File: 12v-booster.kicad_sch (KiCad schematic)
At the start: 21 parts, among them J201 12V_OUT, U202 MPM3810GQB-33, U203 TPS61089RNRR

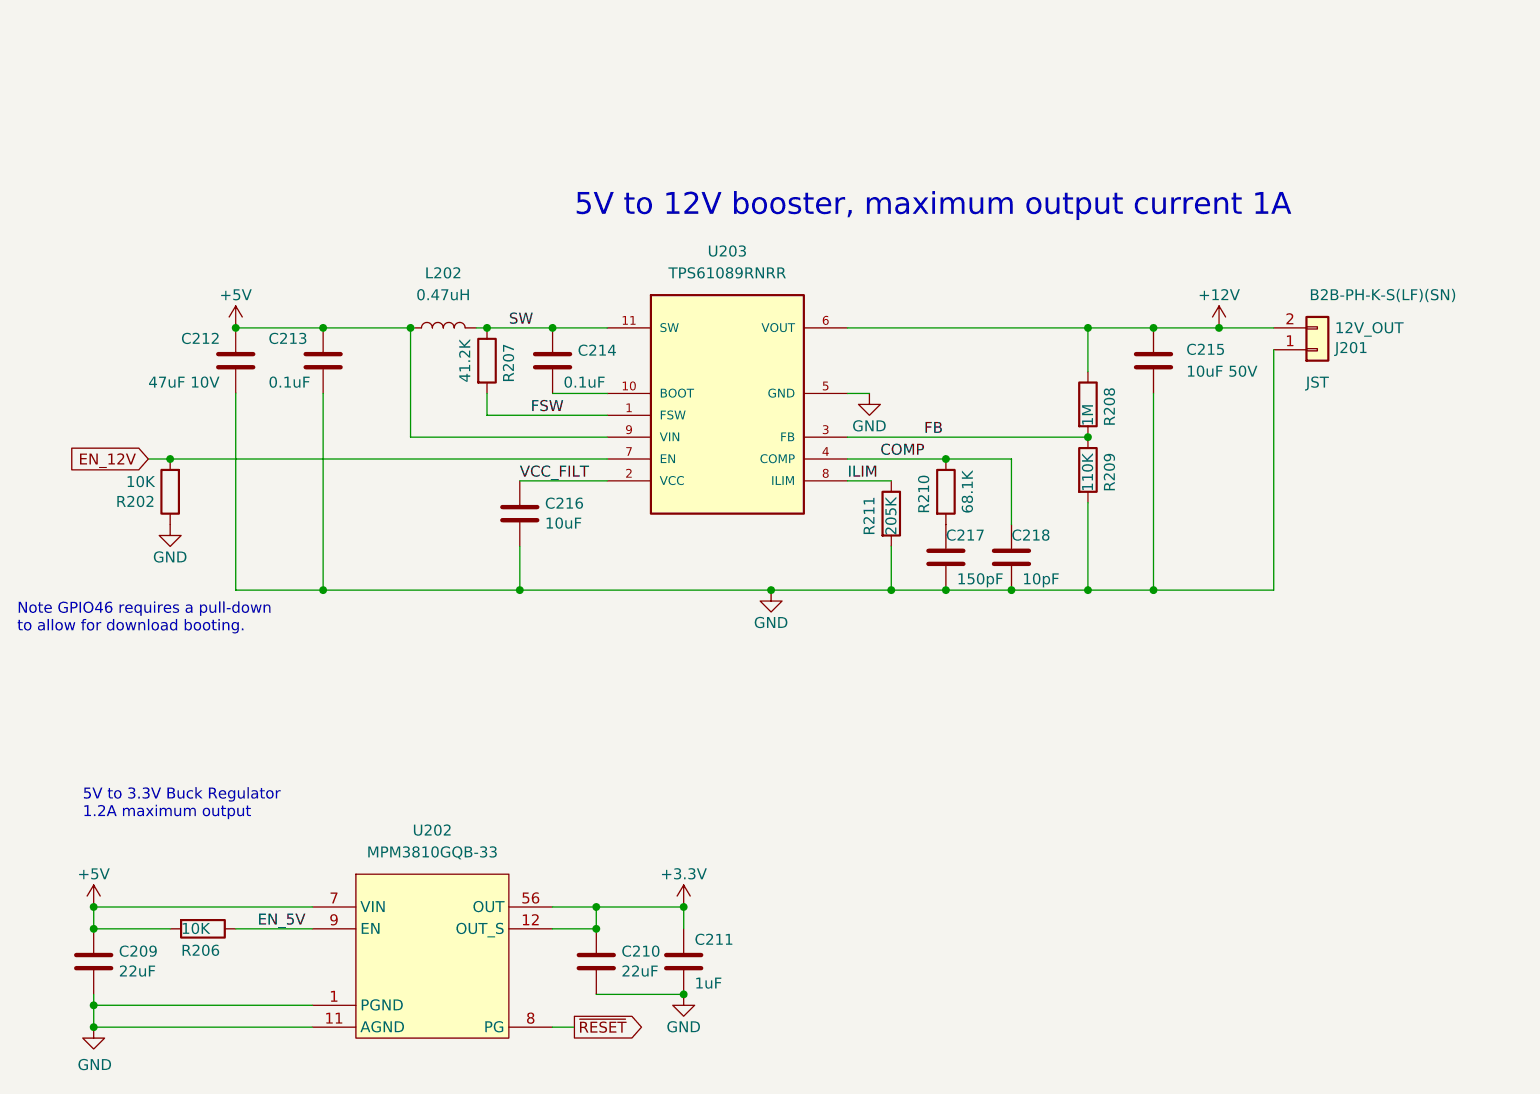
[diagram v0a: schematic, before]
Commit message: Latest 4.0 settings for pcbway
Signed-off-by: Aaron Williams <aaron.w2@gmail.com>
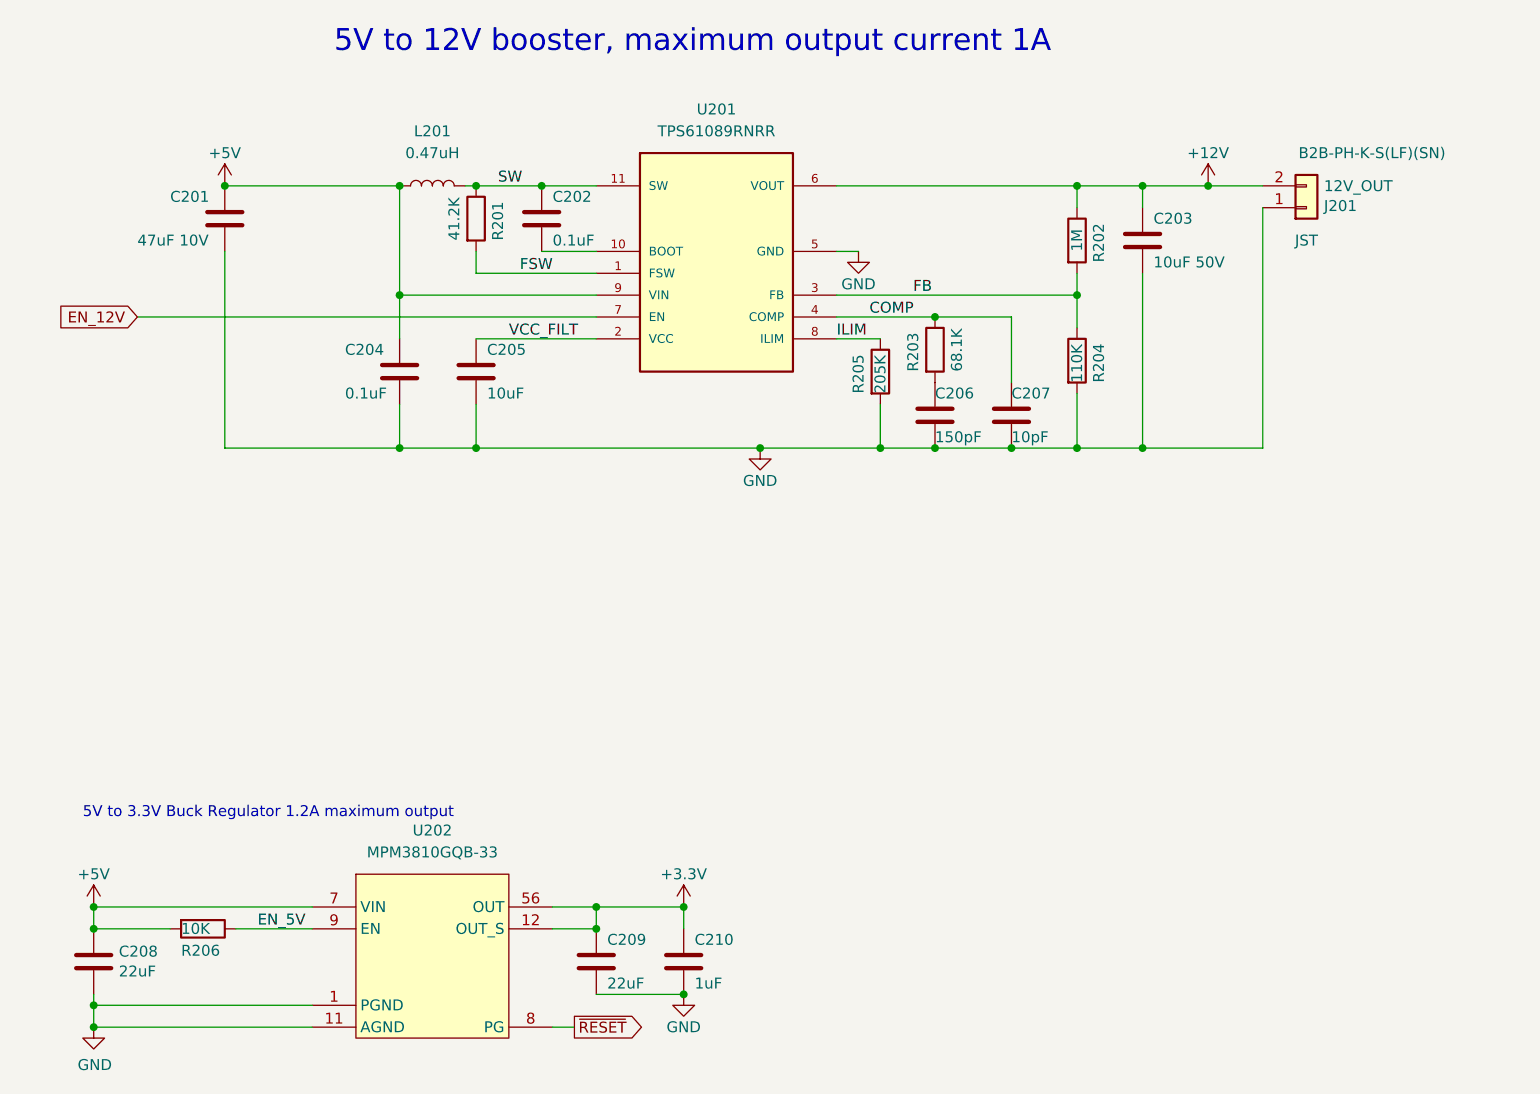
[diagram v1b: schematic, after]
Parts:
- removed R202: 10K, Resistor_SMD:R_0402_1005Metric, symbol Device:R
- C201: renamed from C212; SPN (none) -> 490-9961-1-ND; SPR (none) -> Digikey; SPURL (none) -> https://www.digikey.com/en/products/detail/murata-electroni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
- C203: renamed from C215; MFR (none) -> Murata Electronics; MPN (none) -> GRM21BR61H106KE43L; SPN (none) -> 490-18663-1-ND; SPR (none) -> Digikey; SPURL (none) -> https://www.digikey.com/en/products/detail/murata-electroni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
- C208: renamed from C209; DESC CAP CER 22UF 16V X5R 0603 -> 22 µF ±20% 16V Ceramic Capacitor X5R 0603 (1608 Metric); DK_Datasheet_Link (none) -> https://media.digikey.com/pdf/Data%20Sheets/Samsung%20PDFs/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; DK_Detail_Page (none) -> https://www.digikey.com/en/products/detail/samsung-electro-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; Digi-Key_PN (none) -> 1276-7076-1-ND; MANUFACTURER (none) -> Samsung Electro-Mechanics; Manufacturer (none) -> Samsung Electro-Mechanics; SPURL https://www.digikey.com/products/en/capacitors/ceramic-capa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 -> https://www.digikey.com/en/products/detail/samsung-electro-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
- C209: renamed from C210; DESC CAP CER 22UF 16V X5R 0603 -> 22 µF ±20% 16V Ceramic Capacitor X5R 0603 (1608 Metric); DK_Datasheet_Link (none) -> https://media.digikey.com/pdf/Data%20Sheets/Samsung%20PDFs/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; DK_Detail_Page (none) -> https://www.digikey.com/en/products/detail/samsung-electro-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; Digi-Key_PN (none) -> 1276-7076-1-ND; MANUFACTURER (none) -> Samsung Electro-Mechanics; Manufacturer (none) -> Samsung Electro-Mechanics; SPURL https://www.digikey.com/products/en/capacitors/ceramic-capa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 -> https://www.digikey.com/en/products/detail/samsung-electro-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
- C210: renamed from C211; DESC (none) -> CAP CER 1UF 25V X5R 0402; Digi-Key_PN (none) -> 490-GRM155R61E105MA12JCT-ND; MANUFACTURER (none) -> Murata Electronics; MFR (none) -> Murata Electronics; MPN (none) -> GRM155R61E105MA12J; Manufacturer (none) -> Murata Electronics; Manufacturer Part Number (none) -> GRM155R61E105MA12J; SPN (none) -> 490-GRM155R61E105MA12JCT-ND; SPURL (none) -> https://www.digikey.com/en/products/detail/murata-electroni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
- L201: renamed from L202; DESC (none) -> 470 nH Shielded Drum Core, Wirewound Inductor 7 A 19.2mOhm 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; DK_Datasheet_Link (none) -> https://www.bourns.com/docs/product-datasheets/srp3212.pdf; DK_Detail_Page (none) -> https://www.bourns.com/docs/product-datasheets/srp3212.pdf; Digi-Key_PN (none) -> 118-SRP3212-R47MCT-ND; MFR (none) -> Bourns Inc.; MPN (none) -> SRP3212-R47M; Manufacturer (none) -> Bourns Inc.; Manufacturer Part Number (none) -> SRP3212-R47M; SPN (none) -> 118-SRP3212-R47MCT-ND; SPR (none) -> Digikey; SPURL (none) -> https://www.bourns.com/docs/product-datasheets/srp3212.pdf; Status (none) -> Active
- R201: renamed from R207; SPN 541-2979-1-ND -> (none); SPR Digikey -> (none); SPURL https://www.digikey.com/products/en?keywords=541-2979-1-ND -> (none)
- R204: renamed from R209; DESC 100 kOhms ±1% 0.063W, 1/16W Chip Resistor 0402 (1005 Metric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 -> (none); MFR YAGEO -> (none); MPN RC0402FR-07100KL -> (none); SPN 311-100KLRCT-ND -> (none); SPR Digikey -> (none)
- R206: DESC (none) -> 10 kOhms ±1% 0.063W, 1/16W Chip Resistor 0402 (1005 Metric)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; Digi-Key_PN (none) -> 311-10.0KLRCT-ND; MANUFACTURER (none) -> YAGEO; MFR (none) -> YAGEO; MPN (none) -> RC0402FR-0710KL; Manufacturer (none) -> YAGEO; Manufacturer Part Number (none) -> RC0402FR-0710KL; SPN 541-2979-1-ND -> 311-10.0KLRCT-ND; SPURL https://www.digikey.com/products/en?keywords=541-2979-1-ND -> https://www.digikey.com/en/products/detail/yageo/RC0402FR-0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
- U201: renamed from U203; MFR (none) -> Texas Instruments; MPN (none) -> TPS61089RNRR; SPN (none) -> 296-47295-1-ND; SPR (none) -> Digikey; SPURL (none) -> https://www.digikey.com/en/products/detail/texas-instrument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
- U202: MFR (none) -> Monolithic Power Systems Inc.; MPN (none) -> MPM3810GQB-33-Z; SPN (none) -> 1589-MPM3810GQB-33-ZCT-ND; SPR (none) -> Digikey; SPURL (none) -> https://www.digikey.com/en/products/detail/monolithic-power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
- renumbered C214 to C202, C213 to C204, C216 to C205, C217 to C206, C218 to C207, R208 to R202, R210 to R203, R211 to R205
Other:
- note removed: "Note GPIO46 requires a pull-down to allow for download booting."
- moved on the sheet: C201, C202, C203, C204, C205, C206, C207, J201, L201, R201, R202, R203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
